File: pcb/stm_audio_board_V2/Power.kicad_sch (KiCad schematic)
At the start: 37 parts, among them U2 OP275, U3 MP-K7805-500R3, U4 OP275, U5 MIC2920A-3.3WS-TR, U8 ROHM BA09CC0FP-E2, U9 MIC2920A-3.3WS-TR

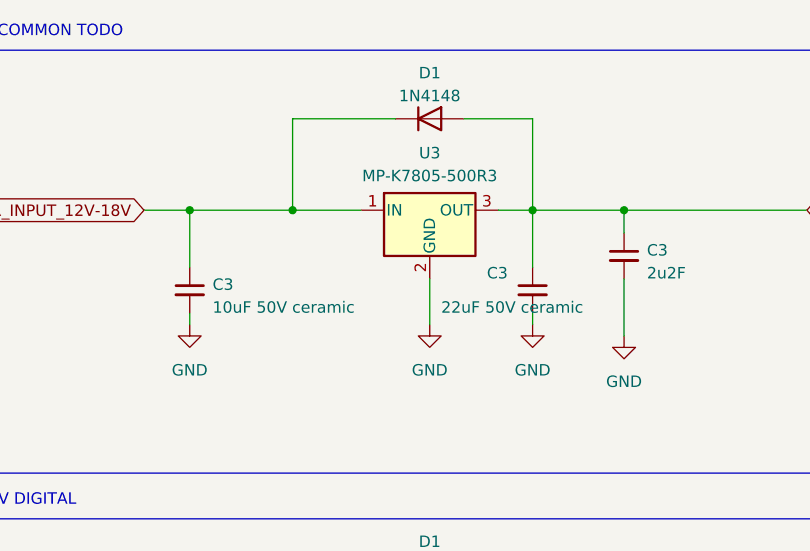
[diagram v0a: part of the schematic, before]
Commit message: pinsetup ready
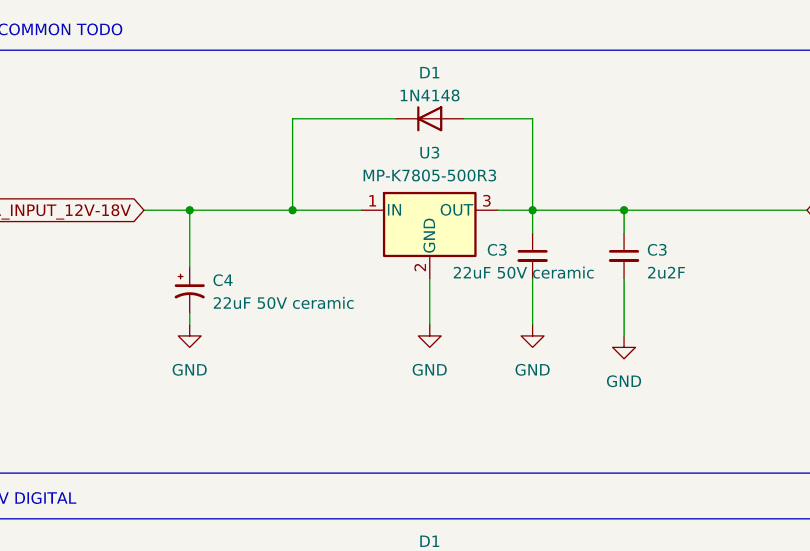
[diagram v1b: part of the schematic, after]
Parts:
- removed C3: 10uF 50V ceramic, Capacitor_SMD:C_0603_1608Metric_Pad1.08x0.95mm_HandSolder, symbol Device:C_Small
- added C4: 22uF 50V ceramic, Capacitor_THT:CP_Radial_D6.3mm_P2.50mm, symbol Device:C_Polarized_Small_US
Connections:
- net GND: now also C4.2
- net PWR_INPUT_12V-18V: now also C4.1
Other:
- moved on the sheet: C3
